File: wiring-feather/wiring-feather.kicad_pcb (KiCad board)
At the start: 2 copper layers, 12 parts, among them J1 M Battery 1, J2 M Battery 1, J3 Screw_Terminal_01x02, J4 Screw_Terminal_01x02, J5 JST Breakout Board, J6 JST Breakout Board, J7 Screw_Terminal_01x02, J8 Screw_Terminal_01x02, J9 JST Breakout Board, U1 TB6612FNG-Breakout, U4 ICM-20948-Adafruit

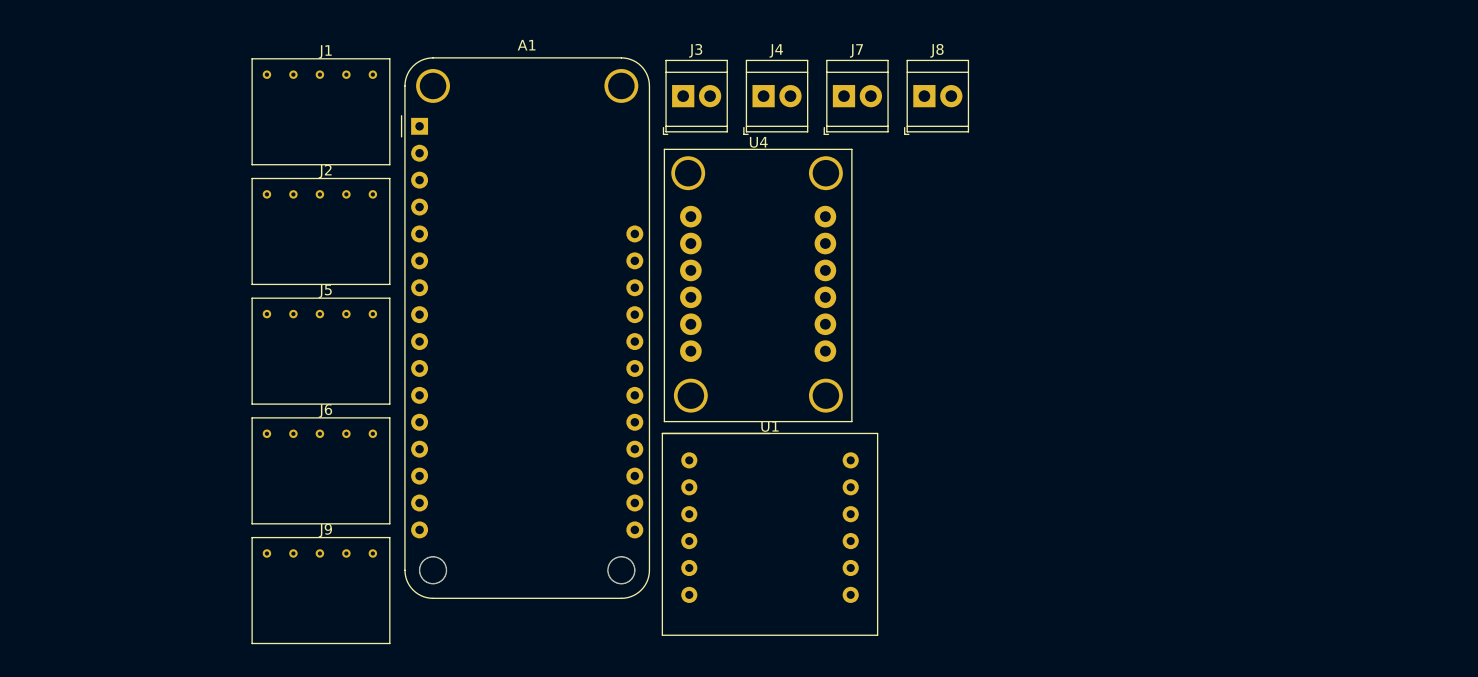
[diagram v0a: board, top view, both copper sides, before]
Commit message: made rough pcb
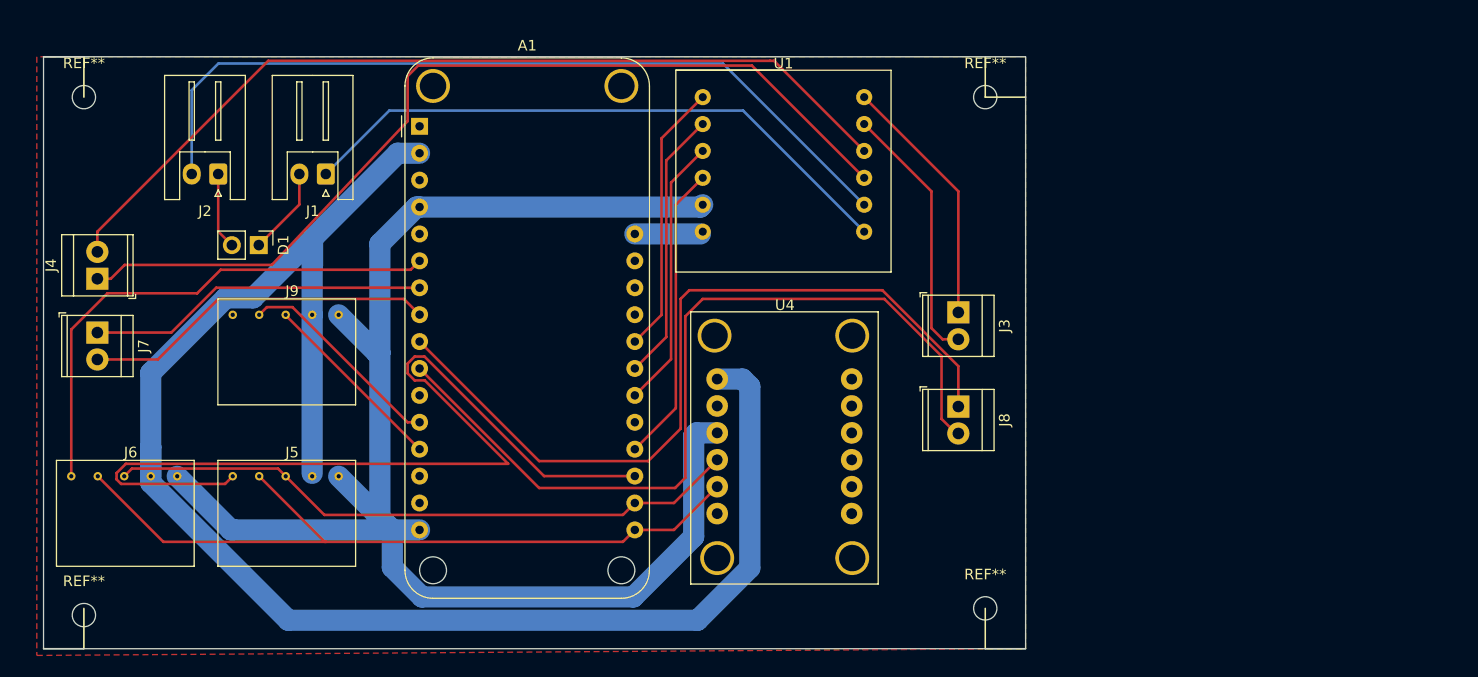
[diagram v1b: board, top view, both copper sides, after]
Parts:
- added D1: D, Connector_PinHeader_2.54mm:PinHeader_1x02_P2.54mm_Vertical, F.Cu at (119.4, 83.8)
- added REF**: MountingHole_2.2mm_M2, MountingHole:MountingHole_2.2mm_M2, F.Cu at (188.0, 118.1)
- added REF**: MountingHole_2.2mm_M2, MountingHole:MountingHole_2.2mm_M2, F.Cu at (102.9, 69.8)
- added REF**: MountingHole_2.2mm_M2, MountingHole:MountingHole_2.2mm_M2, F.Cu at (188.0, 69.8)
- added REF**: MountingHole_2.2mm_M2, MountingHole:MountingHole_2.2mm_M2, F.Cu at (102.9, 118.7)
- J1, J2: footprint 380_footprint-lib:JST_breakout -> Connector_JST:JST_XH_S2B-XH-A_1x02_P2.50mm_Horizontal
- moved J7 73.9 mm to (104.1, 92.1), turned to -90 degrees
- moved J4 65.2 mm to (104.1, 87.0), turned to 90 degrees
- moved U1 34.3 mm to (168.9, 69.8)
- moved J3 33.0 mm to (185.4, 90.2), turned to -90 degrees
- moved J8 29.5 mm to (185.4, 99.1), turned to -90 degrees
- moved J9 22.8 mm to (115.5, 88.9)
- moved J6 18.9 mm to (100.3, 104.1)
- moved J5 15.6 mm to (115.5, 104.1)
- moved U4 15.5 mm to (160.2, 90.1)
- moved J1 12.9 mm to (125.7, 77.1), turned to 180 degrees
- moved J2 3.23 mm to (115.5, 77.1), turned to 180 degrees
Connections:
- A1 pad 19: /PWM-M1 -> /RESET
- A1 pad 20: /DIR1-M1 -> /DIR1-M2
- A1 pad 23: /DIR1-M2 -> /PWM-M1
- A1 pad 24: /RESET -> /DIR1-M1
- J1 pad 1: Net-(D1-K) -> /BATT+
- J1 pad 2: /BATT+ -> Net-(D1-K)
- J2 pad 1: /BATT_ -> Net-(D1-A)
- J2 pad 2: Net-(D1-A) -> /BATT_
- J4 pad 1: /PWR_M2 -> /NEG_M2
- J4 pad 2: /NEG_M2 -> /PWR_M2
- U1 pad 5: unconnected-(U1-GND-Pad5) -> GND
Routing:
- net +3V3: track 0.00 -> 160.4 mm
- net GND: track 0.00 -> 144.4 mm
- net /RESET: track 0.00 -> 89.7 mm
- net /NEG_M2: track 0.00 -> 87.8 mm
- net /PWR_M2: track 0.00 -> 84.5 mm
- net /ENCB_M1: track 0.00 -> 80.6 mm
- net /BATT_: track 0.00 -> 78.0 mm
- net /ENCA_M1: track 0.00 -> 76.2 mm
- net /SDA: track 0.00 -> 72.1 mm
- net /SCL: track 0.00 -> 60.5 mm
- net /BATT+: track 0.00 -> 58.0 mm
- net /INT: track 0.00 -> 49.4 mm
- net /ENCA_M2: track 0.00 -> 33.4 mm
- net /ENCB_M2: track 0.00 -> 32.2 mm
- net /DIR1-M2: track 0.00 -> 28.3 mm
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- added copper zone on F.Cu, net GND
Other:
- board outline added: 92.7 x 55.9 mm

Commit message: updated pcb
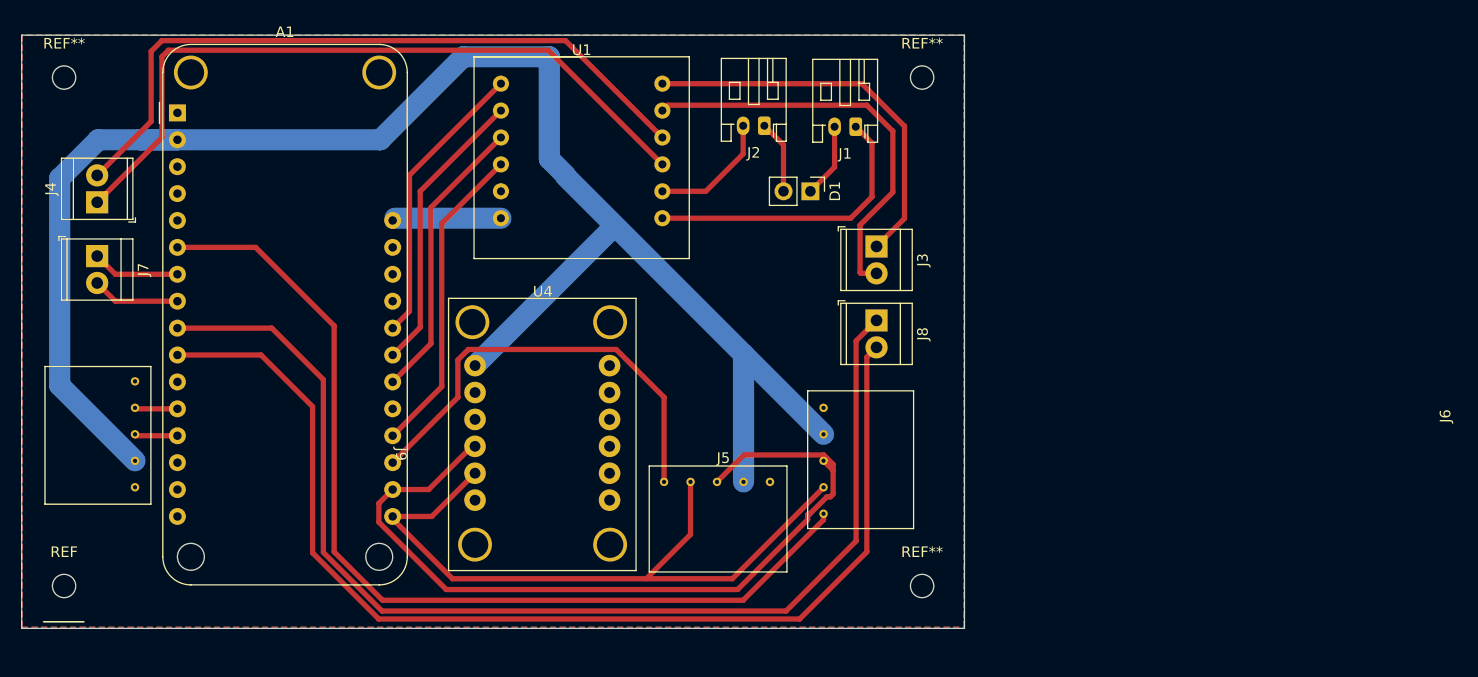
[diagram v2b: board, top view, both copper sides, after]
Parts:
- J1, J2: footprint Connector_JST:JST_XH_S2B-XH-A_1x02_P2.50mm_Horizontal -> Connector_JST:JST_PH_S2B-PH-K_1x02_P2.00mm_Horizontal
- moved J6 71.2 mm to (171.2, 110.6), turned to 90 degrees
- moved D1 52.3 mm to (171.5, 78.7)
- moved J2 51.8 mm to (167.1, 72.6)
- moved J1 50.2 mm to (175.7, 72.6)
- moved J5 40.7 mm to (156.2, 104.7)
- moved U4 22.9 mm to (137.3, 88.8)
- moved A1 22.9 mm to (111.7, 71.3)
- moved U1 19.1 mm to (149.9, 68.6)
- moved J8 11.2 mm to (177.7, 90.9)
- moved J3 9.92 mm to (177.7, 83.9)
- moved J9 8.98 mm to (109.2, 95.3), turned to -90 degrees
- moved J4 7.22 mm to (104.1, 79.8)
- moved J7 7.22 mm to (104.1, 84.9)
- moved REF** 6.32 mm to (182.0, 116.0)
- moved REF** 6.24 mm to (182.0, 68.0)
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- renumbered REF** to REF
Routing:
- net GND: track 144.4 -> 0.00 mm
- net /BATT_: track 78.0 -> 11.7 mm
- net /RESET: track 89.7 -> 42.0 mm
- net /INT: track 49.4 -> 91.0 mm
- net /ENCA_M1: track 76.2 -> 109.0 mm
- net /BATT+: track 58.0 -> 27.9 mm
- net /ENCB_M1: track 80.6 -> 105.8 mm
- net /ENCA_M2: track 33.4 -> 8.29 mm
- net /ENCB_M2: track 32.2 -> 8.29 mm
- net /NEG_M2: track 87.8 -> 68.2 mm
- net /SCL: track 60.5 -> 79.1 mm
- net /PWR_M2: track 84.5 -> 66.3 mm
- net /SDA_2: track 19.9 -> 4.04 mm
- net /NEG_M1: track 24.9 -> 39.2 mm
- net /SCL_2: track 17.9 -> 4.06 mm
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- added copper zone on B.Cu, net GND
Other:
- board size 92.7 x 55.9 mm -> 89 x 56 mm
